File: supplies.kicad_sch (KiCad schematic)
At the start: 29 parts, among them J19 KEY_SWITCH, U16 L7805, U17 AMS1117-3.3

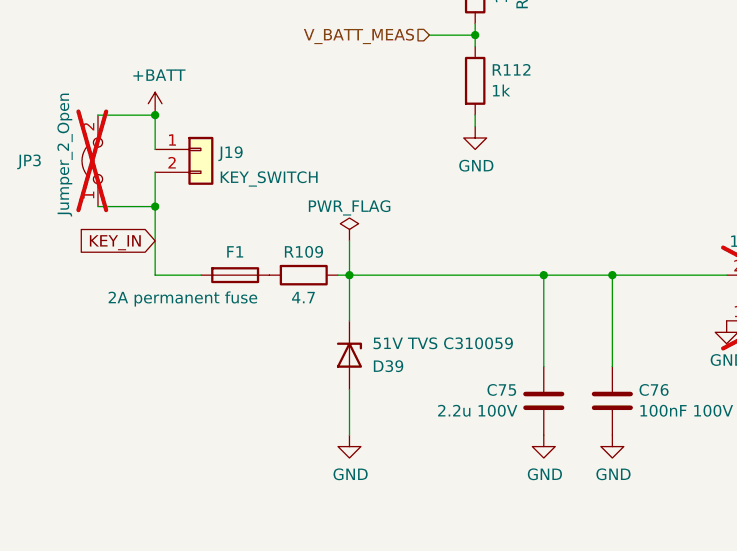
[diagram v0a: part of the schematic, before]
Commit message: update lcsc numbers
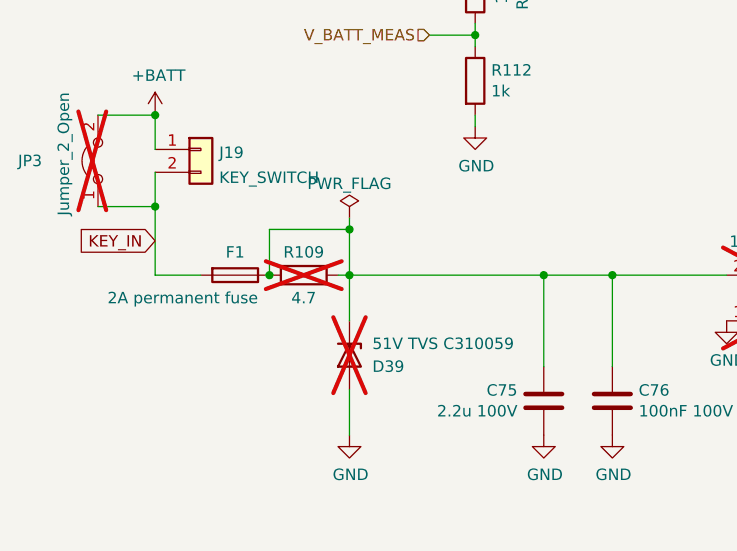
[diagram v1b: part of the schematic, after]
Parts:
- C75, C80: place hand -> (none)
- D39, R109: now not fitted; now left out of the parts list
- F1: LCSC C182310 -> C99538
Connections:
- net at C75.1, C76.1, D39.1 (K)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: now also F1.1, R109.2
